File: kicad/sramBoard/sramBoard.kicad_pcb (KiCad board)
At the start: 4 copper layers, 180 x 180 mm, 1225 parts, among them J1 Conn_02x20_Top_Bottom, Q1 NMOS, Q10 NMOS, Q100 NMOS, Q1000 NMOS, Q1001 NMOS, Q1002 NMOS, Q1003 PMOS, Q1004 NMOS, Q1005 PMOS, Q1006 NMOS, Q1007 NMOS, Q1008 NMOS, Q1009 NMOS, Q101 PMOS, Q1010 NMOS, Q1011 PMOS, Q1012 NMOS, Q1013 PMOS, Q1014 NMOS, Q1015 NMOS, Q1016 NMOS, Q1017 NMOS, Q1018 NMOS, Q1019 PMOS, Q102 NMOS, Q1020 NMOS, Q1021 PMOS, Q1022 NMOS, Q1023 NMOS, Q1024 NMOS, Q1025 PMOS, Q1026 NMOS, Q1027 PMOS, Q1028 NMOS, Q1029 PMOS, Q103 NMOS, Q1030 NMOS, Q1031 PMOS, Q1032 NMOS, Q1033 PMOS, Q1034 PMOS, Q1035 PMOS, Q1036 PMOS, Q1037 PMOS, Q1038 NMOS, Q1039 NMOS, Q104 NMOS, Q1040 NMOS, Q1041 NMOS, Q1042 NMOS, Q1043 PMOS, Q1044 PMOS, Q1045 PMOS, Q1046 PMOS, Q1047 PMOS, Q1048 NMOS, Q1049 NMOS, Q105 NMOS, Q1050 NMOS, Q1051 NMOS, Q1052 NMOS, Q1053 PMOS, Q1054 PMOS, Q1055 PMOS, Q1056 PMOS, Q1057 PMOS, Q1058 NMOS, Q1059 NMOS, Q106 NMOS, Q1060 NMOS, Q1061 NMOS, Q1062 NMOS, Q1063 PMOS, Q1064 PMOS, Q1065 PMOS, Q1066 PMOS, Q1067 PMOS, Q1068 NMOS, Q1069 NMOS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

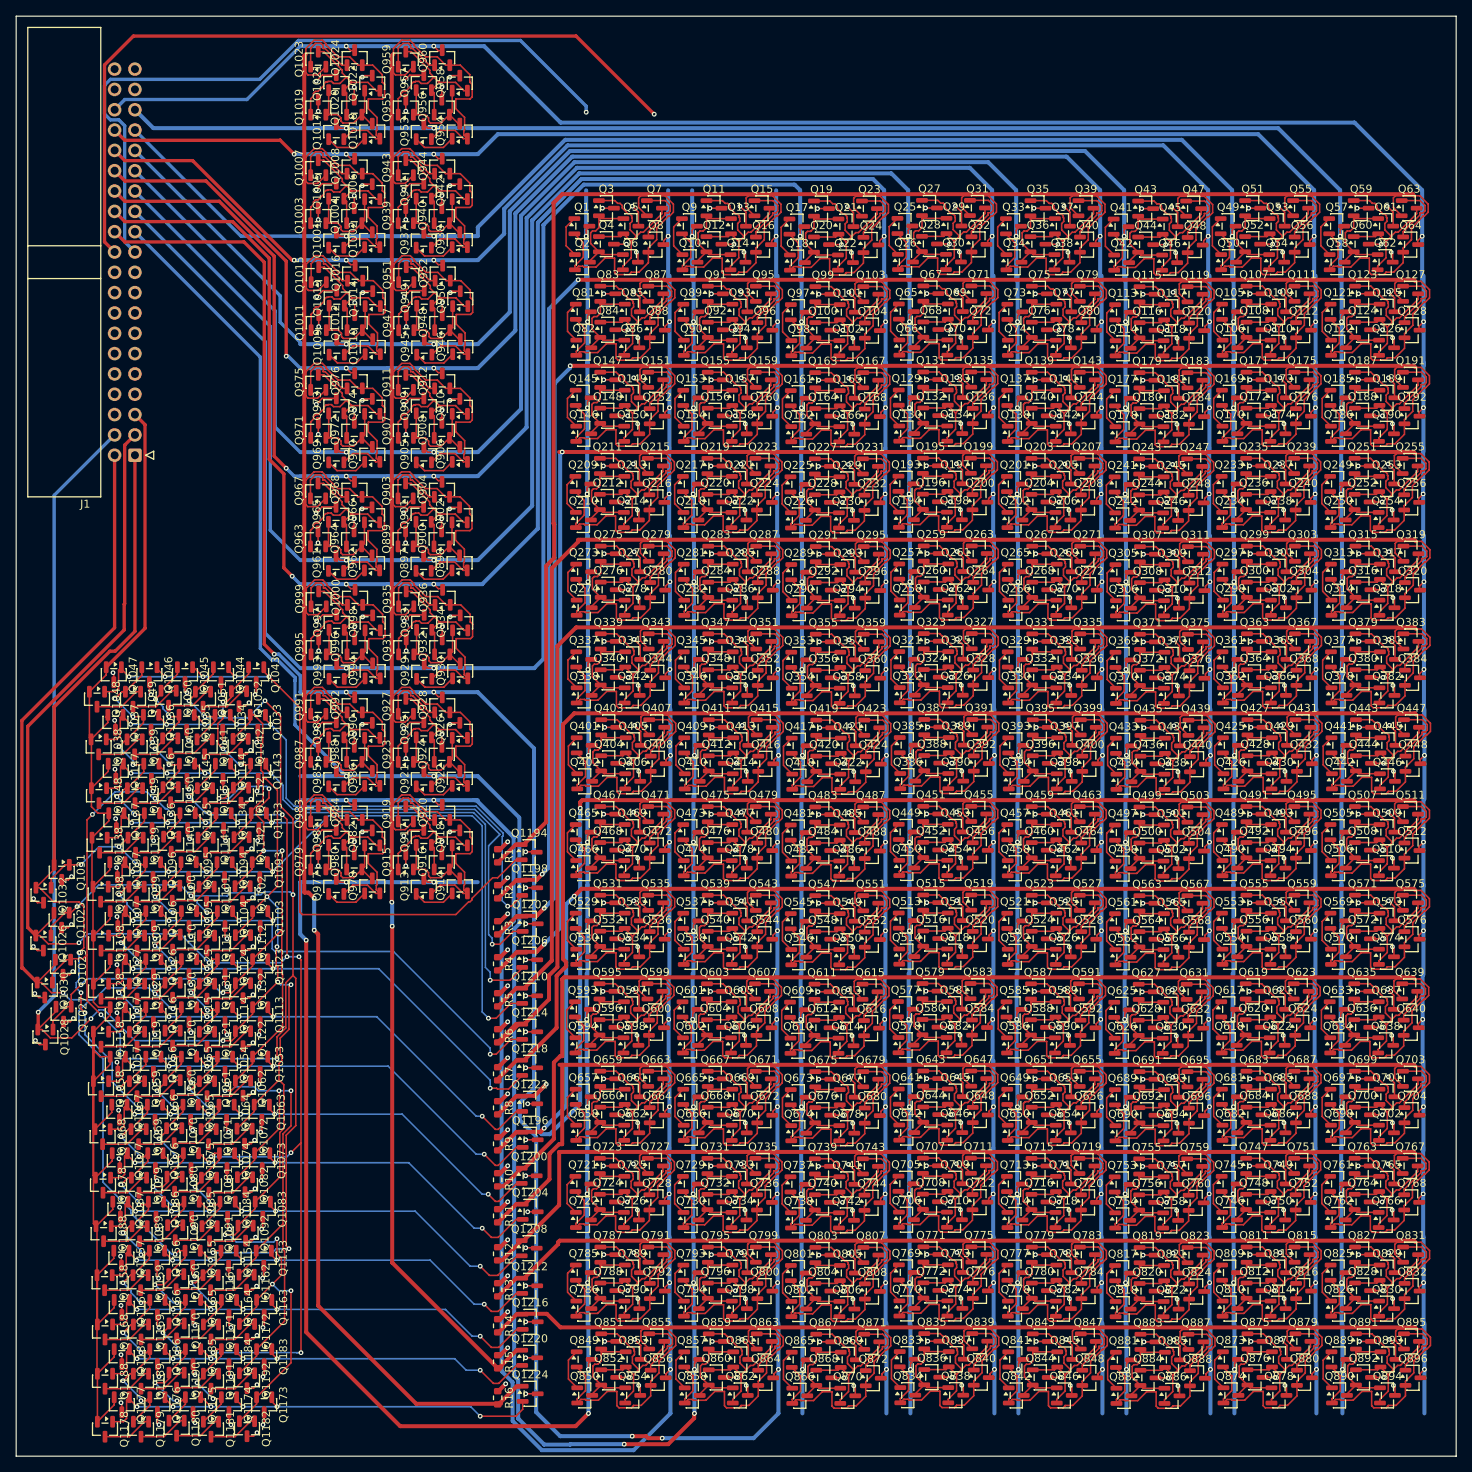
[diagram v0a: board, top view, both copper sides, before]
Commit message: improve pcb labeling
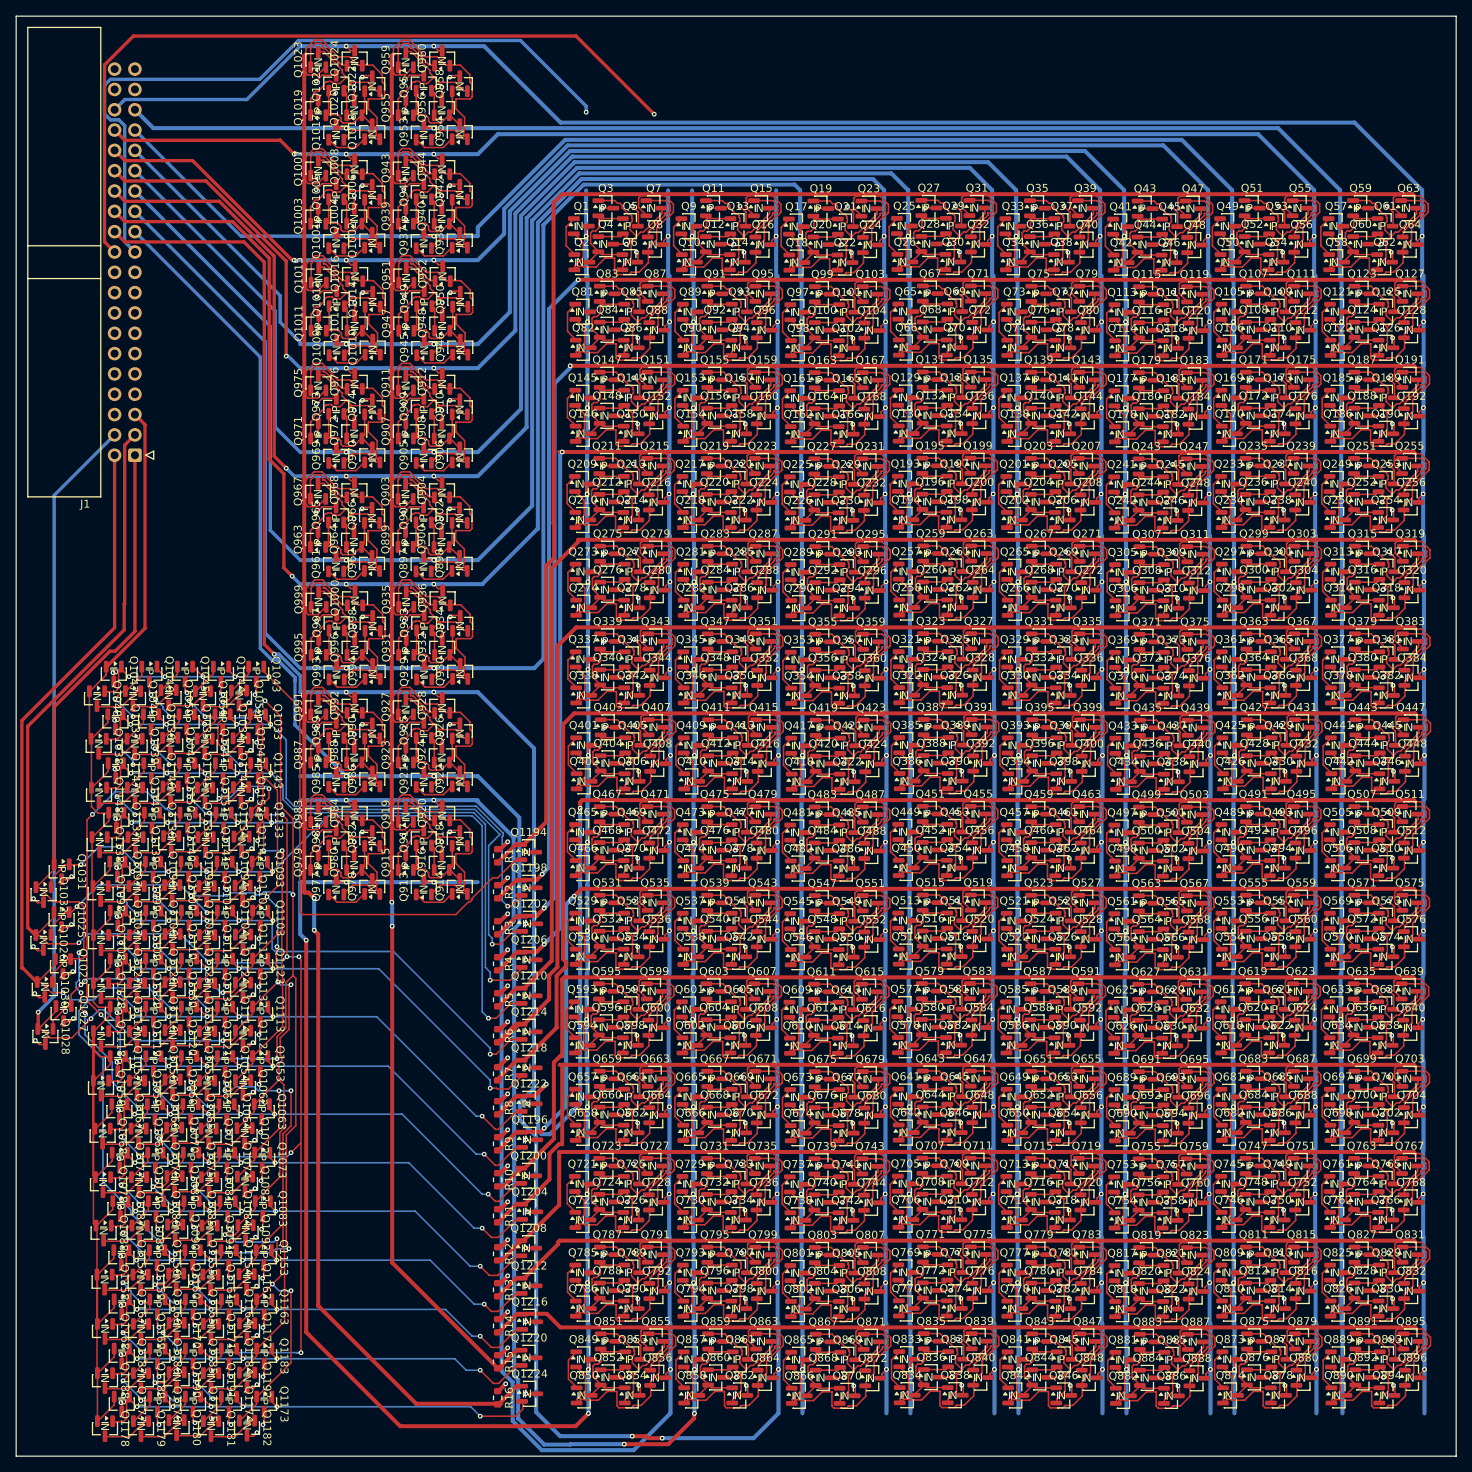
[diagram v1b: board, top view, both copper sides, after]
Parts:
- Q1, Q10, Q100, Q1000, Q1001, Q1002, Q1004, Q1006, Q1007, Q1008, Q1009, Q1010, Q1012, Q1014, Q1015, Q1016, Q1017, Q1018, Q102, Q1020, Q1022, Q1023, Q1024, Q1026, Q1028, Q103, Q1030, Q1032, Q1038, Q1039, Q104, Q1040, Q1041, Q1042, Q1048, Q1049, Q105, Q1050, Q1051, Q1052, Q1058, Q1059, Q106, Q1060, Q1061, Q1062, Q1068, Q1069, Q1070, Q1071, Q1072, Q1078, Q1079, Q108, Q1080, Q1081, Q1082, Q1088, Q1089, Q1090, Q1091, Q1092, Q1098, Q1099, Q110, Q1100, Q1101, Q1102, Q1108, Q1109, Q111, Q1110, Q1111, Q1112, Q1118, Q1119, Q112, Q1120, Q1121, Q1122, Q1128, Q1129, Q113, Q1130, Q1131, Q1132, Q1138, Q1139, Q114, Q1140, Q1141, Q1142, Q1148, Q1149, Q1150, Q1151, Q1152, Q1158, Q1159, Q116, Q1160, Q1161, Q1162, Q1168, Q1169, Q1170, Q1171, Q1172, Q1178, Q1179, Q118, Q1180, Q1181, Q1182, Q1188, Q1189, Q119, Q1190, Q1191, Q1192, Q1194, Q1196, Q1198, Q12, Q120, Q1200, Q1202, Q1204, Q1206, Q1208, Q121, Q1210, Q1212, Q1214, Q1216, Q1218, Q122, Q1220, Q1222, Q1224, Q124, Q126, Q127, Q128, Q129, Q130, Q132, Q134, Q135, Q136, Q137, Q138, Q14, Q140, Q142, Q143, Q144, Q145, Q146, Q148, Q15, Q150, Q151, Q152, Q153, Q154, Q156, Q158, Q159, Q16, Q160, Q161, Q162, Q164, Q166, Q167, Q168, Q169, Q17, Q170, Q172, Q174, Q175, Q176, Q177, Q178, Q18, Q180, Q182, Q183, Q184, Q185, Q186, Q188, Q190, Q191, Q192, Q193, Q194, Q196, Q198, Q199, Q2, Q20, Q200, Q201, Q202, Q204, Q206, Q207, Q208, Q209, Q210, Q212, Q214, Q215, Q216, Q217, Q218, Q22, Q220, Q222, Q223, Q224, Q225, Q226, Q228, Q23, Q230, Q231, Q232, Q233, Q234, Q236, Q238, Q239, Q24, Q240, Q241, Q242, Q244, Q246, Q247, Q248, Q249, Q25, Q250, Q252, Q254, Q255, Q256, Q257, Q258, Q26, Q260, Q262, Q263, Q264, Q265, Q266, Q268, Q270, Q271, Q272, Q273, Q274, Q276, Q278, Q279, Q28, Q280, Q281, Q282, Q284, Q286, Q287, Q288, Q289, Q290, Q292, Q294, Q295, Q296, Q297, Q298, Q30, Q300, Q302, Q303, Q304, Q305, Q306, Q308, Q31, Q310, Q311, Q312, Q313, Q314, Q316, Q318, Q319, Q32, Q320, Q321, Q322, Q324, Q326, Q327, Q328, Q329, Q33, Q330, Q332, Q334, Q335, Q336, Q337, Q338, Q34, Q340, Q342, Q343, Q344, Q345, Q346, Q348, Q350, Q351, Q352, Q353, Q354, Q356, Q358, Q359, Q36, Q360, Q361, Q362, Q364, Q366, Q367, Q368, Q369, Q370, Q372, Q374, Q375, Q376, Q377, Q378, Q38, Q380, Q382, Q383, Q384, Q385, Q386, Q388, Q39, Q390, Q391, Q392, Q393, Q394, Q396, Q398, Q399, Q4, Q40, Q400, Q401, Q402, Q404, Q406, Q407, Q408, Q409, Q41, Q410, Q412, Q414, Q415, Q416, Q417, Q418, Q42, Q420, Q422, Q423, Q424, Q425, Q426, Q428, Q430, Q431, Q432, Q433, Q434, Q436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: footprint Package_TO_SOT_SMD:SOT-23 -> easyeda2kicad:SOT-23-N
- Q1003, Q1005, Q101, Q1011, Q1013, Q1019, Q1021, Q1025, Q1027, Q1029, Q1031, Q1033, Q1034, Q1035, Q1036, Q1037, Q1043, Q1044, Q1045, Q1046, Q1047, Q1053, Q1054, Q1055, Q1056, Q1057, Q1063, Q1064, Q1065, Q1066, Q1067, Q107, Q1073, Q1074, Q1075, Q1076, Q1077, Q1083, Q1084, Q1085, Q1086, Q1087, Q109, Q1093, Q1094, Q1095, Q1096, Q1097, Q11, Q1103, Q1104, Q1105, Q1106, Q1107, Q1113, Q1114, Q1115, Q1116, Q1117, Q1123, Q1124, Q1125, Q1126, Q1127, Q1133, Q1134, Q1135, Q1136, Q1137, Q1143, Q1144, Q1145, Q1146, Q1147, Q115, Q1153, Q1154, Q1155, Q1156, Q1157, Q1163, Q1164, Q1165, Q1166, Q1167, Q117, Q1173, Q1174, Q1175, Q1176, Q1177, Q1183, Q1184, Q1185, Q1186, Q1187, Q123, Q125, Q13, Q131, Q133, Q139, Q141, Q147, Q149, Q155, Q157, Q163, Q165, Q171, Q173, Q179, Q181, Q187, Q189, Q19, Q195, Q197, Q203, Q205, Q21, Q211, Q213, Q219, Q221, Q227, Q229, Q235, Q237, Q243, Q245, Q251, Q253, Q259, Q261, Q267, Q269, Q27, Q275, Q277, Q283, Q285, Q29, Q291, Q293, Q299, Q3, Q301, Q307, Q309, Q315, Q317, Q323, Q325, Q331, Q333, Q339, Q341, Q347, Q349, Q35, Q355, Q357, Q363, Q365, Q37, Q371, Q373, Q379, Q381, Q387, Q389, Q395, Q397, Q403, Q405, Q411, Q413, Q419, Q421, Q427, Q429, Q43, Q435, Q437, Q443, Q445, Q45, Q451, Q453, Q459, Q461, Q467, Q469, Q475, Q477, Q483, Q485, Q491, Q493, Q499, Q5, Q501, Q507, Q509, Q51, Q515, Q517, Q523, Q525, Q53, Q531, Q533, Q539, Q541, Q547, Q549, Q555, Q557, Q563, Q565, Q571, Q573, Q579, Q581, Q587, Q589, Q59, Q595, Q597, Q603, Q605, Q61, Q611, Q613, Q619, Q621, Q627, Q629, Q635, Q637, Q643, Q645, Q651, Q653, Q659, Q661, Q667, Q669, Q67, Q675, Q677, Q683, Q685, Q69, Q691, Q693, Q699, Q701, Q707, Q709, Q715, Q717, Q723, Q725, Q731, Q733, Q739, Q741, Q747, Q749, Q75, Q755, Q757, Q763, Q765, Q77, Q771, Q773, Q779, Q781, Q787, Q789, Q795, Q797, Q803, Q805, Q811, Q813, Q819, Q821, Q827, Q829, Q83, Q835, Q837, Q843, Q845, Q85, Q851, Q853, Q859, Q861, Q867, Q869, Q875, Q877, Q883, Q885, Q891, Q893, Q899, Q901, Q907, Q909, Q91, Q915, Q917, Q923, Q925, Q93, Q931, Q933, Q939, Q941, Q947, Q949, Q955, Q957, Q963, Q965, Q971, Q973, Q979, Q981, Q987, Q989, Q99, Q995, Q997: footprint Package_TO_SOT_SMD:SOT-23 -> easyeda2kicad:SOT-23-P
